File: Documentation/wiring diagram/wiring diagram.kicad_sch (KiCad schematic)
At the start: 3 parts, among them SW1 SW_Push_DPDT, SW2 SW_Push_DPDT

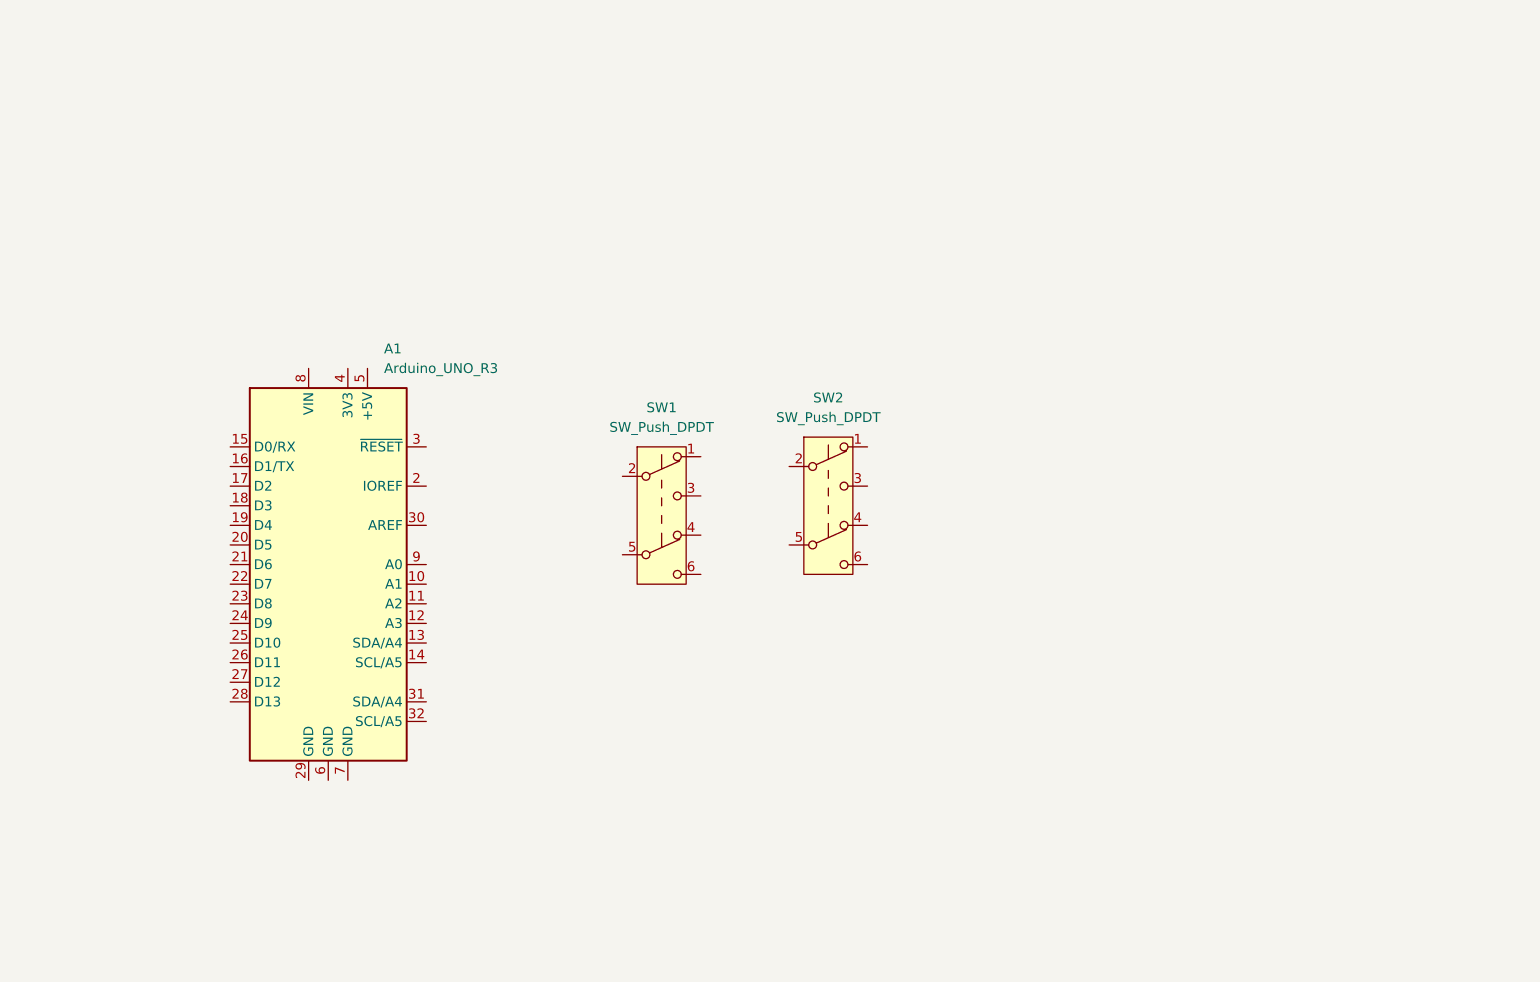
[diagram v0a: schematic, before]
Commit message: updated changes to wiring diagram
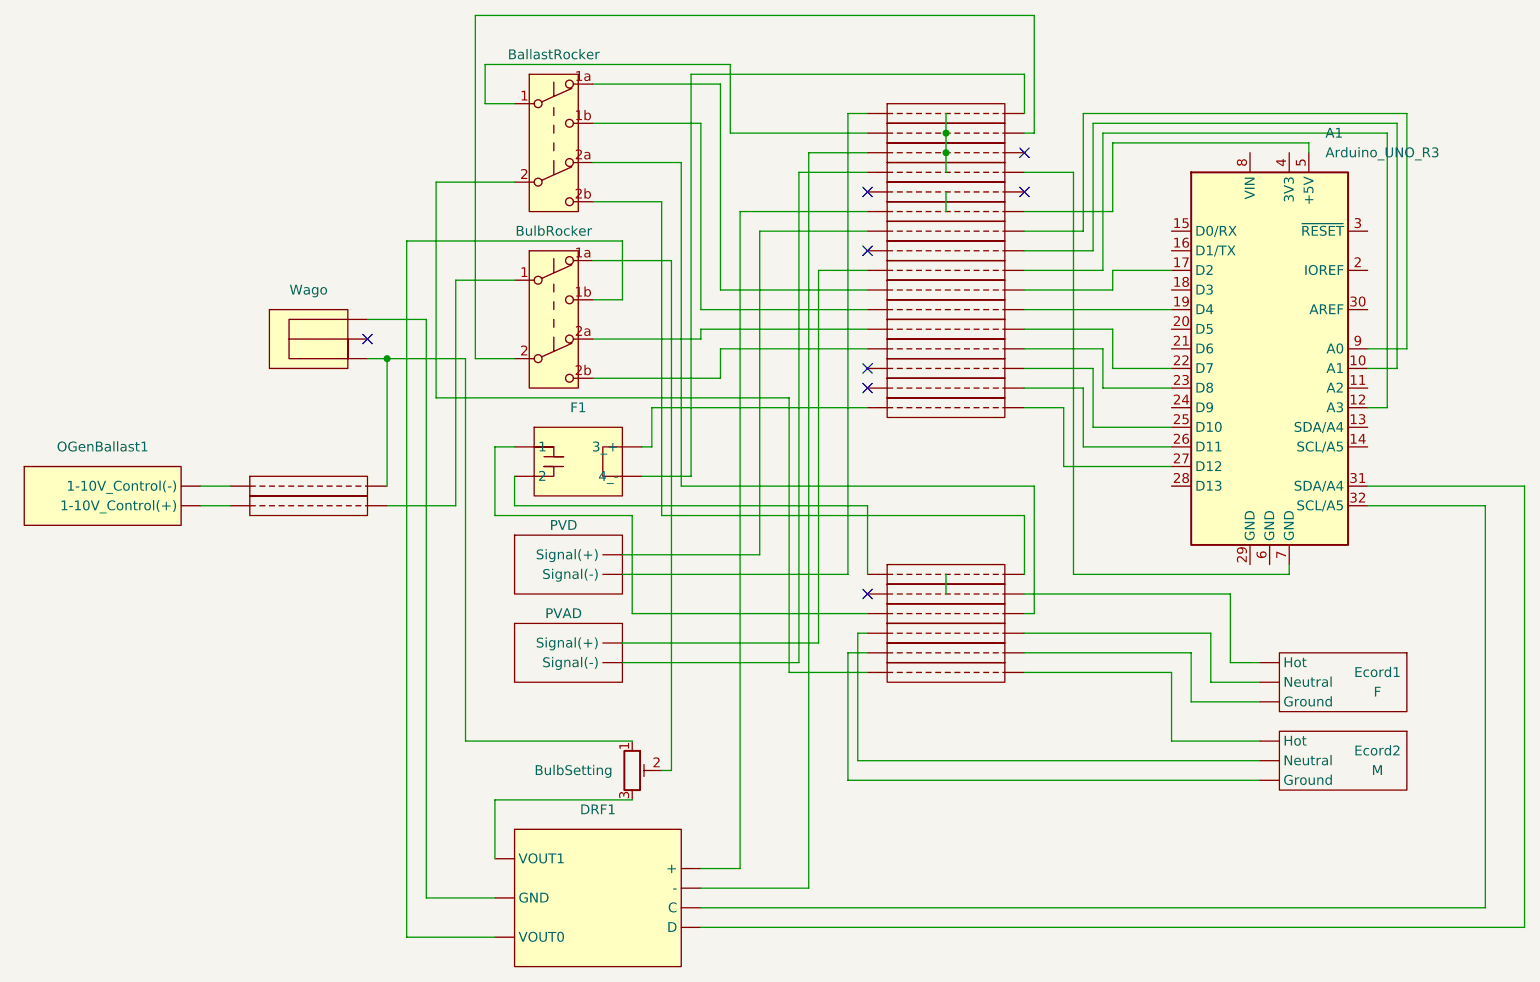
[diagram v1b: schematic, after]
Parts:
- removed SW2: SW_Push_DPDT, symbol Switch:SW_Push_DPDT
- added BulbRocker: SW_Push_DPDT, symbol Switch:SW_Push_DPDT
- added BulbSetting: R_Potentiometer_Trim, symbol Device:R_Potentiometer_Trim
- added DRF1: (no value), symbol SOYFACE_wiringdiagram_library:DRF0971
- added Ecord1: F, symbol SOYFACE_wiringdiagram_library:Extension_Cord
- added Ecord2: M, symbol SOYFACE_wiringdiagram_library:Extension_Cord
- added F1: (no value), symbol SOYFACE_wiringdiagram_library:Fuse
- added OGenBallast1: (no value), symbol SOYFACE_wiringdiagram_library:Ozone_Generator_Ballast
- added PVAD, PVD: O1, symbol SOYFACE_wiringdiagram_library:PVD
- added U1: 1, symbol SOYFACE_wiringdiagram_library:BUS
- added U10, U11, U12, U13, U14, U15, U16, U17, U18, U19, U2, U20, U21, U22, U23, U24, U3, U4, U5, U6, U7, U8, U9: 2, symbol SOYFACE_wiringdiagram_library:BUS
- added Wago: (no value), symbol SOYFACE_wiringdiagram_library:WAGO
- renumbered SW1 to BallastRocker
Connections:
- net at BallastRocker.1 (B): now also U15.
- net at BallastRocker.2 (B): now also U24.
- net at A1.10 (A1): now also U9.
- net at A1.12 (A3): now also U8.
- net at A1.17 (D2): now also U1.
- net at A1.19 (D4): now also U2.
- net at A1.22 (D7): now also U3.
- net at A1.23 (D8): now also U4.
- net at A1.25 (D10): now also U5.
- net at A1.26 (D11): now also U6.
- net at A1.27 (D12): now also U7.
- net at A1.31 (SDA/A4): now also DRF1. (D)
- net at A1.32 (SCL/A5): now also DRF1. (D)
- net at A1.5 (+5V): now also U11.
- net at A1.7 (GND): now also U13.
- net at A1.9 (A0): now also U10.
- new net: BallastRocker.1a (A), U1.
- new net: BulbRocker.2b (C), U4.
- new net: OGenBallast1. (1-10V_Control(+)), U18.
- new net: BulbRocker.1 (B), U18.
- new net: DRF1. (D), Wago.
- new net: DRF1. (D), U14.
- new net: DRF1. (D), U11.
- new net: BulbSetting.3, DRF1. (D)
- new net: BulbRocker.1b (C), DRF1. (D)
- new net: PVD. (Signal(-)), U10.
- new net: U11., U12.
- new net: PVD. (Signal(-)), U16.
- new net: Ecord2. (Ground), U24.
- new net: BallastRocker.2a (A), U21.
- new net: F1. (4_-), U21.
- new net: Ecord2. (Ground), U22.
- new net: Ecord2. (Ground), U23.
- new net: Ecord1. (Ground), U22.
- new net: PVAD. (Signal(-)), U13.
- new net: U13., U14., U15., U16.
- new net: F1. (4_-), U7.
- new net: Ecord1. (Ground), U23.
- new net: BallastRocker.1b (C), U2.
- new net: BallastRocker.2b (C), U19.
- new net: F1. (4_-), U16.
- new net: F1. (4_-), U19.
- new net: PVAD. (Signal(-)), U8.
- new net: BulbSetting.1, U17., Wago.
- new net: BulbRocker.2a (A), U3.
- new net: OGenBallast1. (1-10V_Control(+)), U17.
- new net: Ecord1. (Ground), U20.
- new net: BulbRocker.2 (B), U15.
- new net: U19., U20.
- new net: BulbRocker.1a (A), BulbSetting.2
- no-connect marks 0 -> 8
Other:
- moved on the sheet: A1, BallastRocker
